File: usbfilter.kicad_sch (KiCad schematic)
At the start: 7 parts, among them U12 USBLC6-2P6

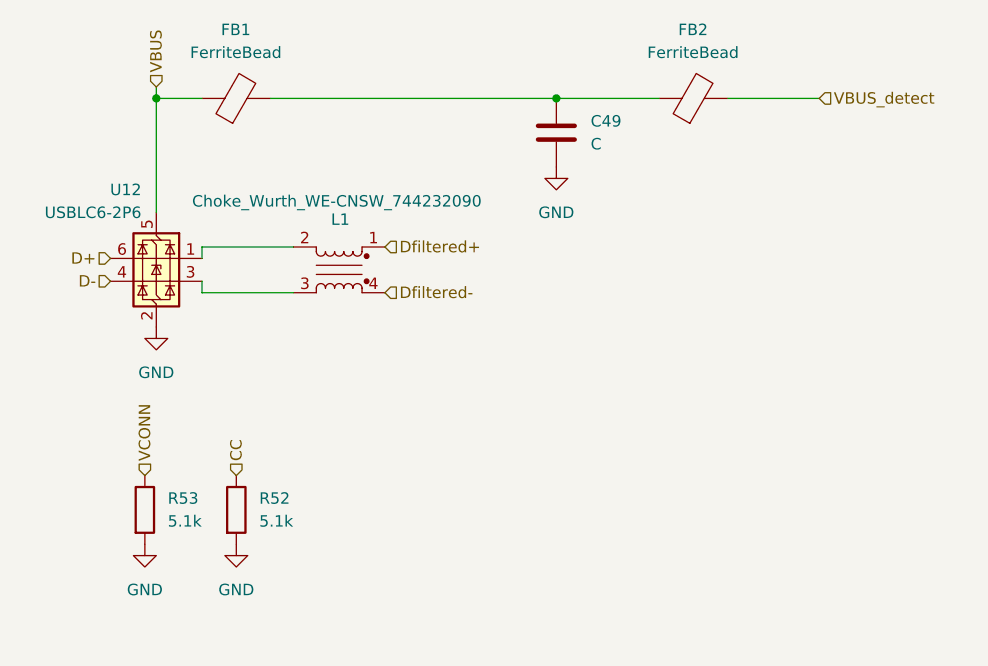
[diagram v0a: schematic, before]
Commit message: modified:   MCU.kicad_sch 	modified:   PSU.kicad_sch 	modified:   ProjectY.kicad_pro 	modified:   ProjectY.kicad_sch 	modified:   audio.kicad_sch 	modified:   fp-info-cache 	new file:   spdif.kicad_sch 	modified:   usbfilter.kicad_sch
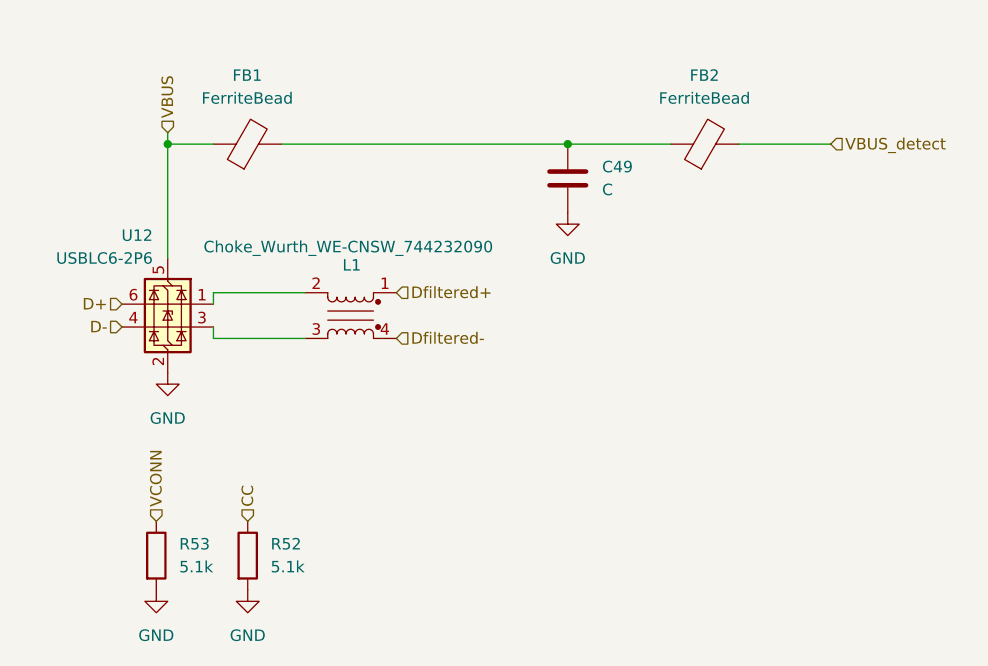
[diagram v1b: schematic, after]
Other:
- moved on the sheet: C49, FB1, FB2, L1, R52, R53, U12
